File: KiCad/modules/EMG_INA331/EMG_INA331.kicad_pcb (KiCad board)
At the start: 4 copper layers, 15 x 11 mm, 47 parts, among them J1 Conn_01x01_Pin, J10 Conn_01x01_Pin, J2 Conn_01x01_Pin, J3 Conn_01x01_Pin, J4 Conn_01x01_Pin, J5 Conn_01x01_Pin, J6 Conn_01x01_Pin, J7 Conn_01x01_Pin, J8 Conn_01x01_Pin, J9 Conn_01x01_Pin, U1 INA350ABSIDSGR, U2 OPA333, U3 AP2112K-3.3TRG1, U4 OPA333, U5 CJ432, U6 LIS3DHTR

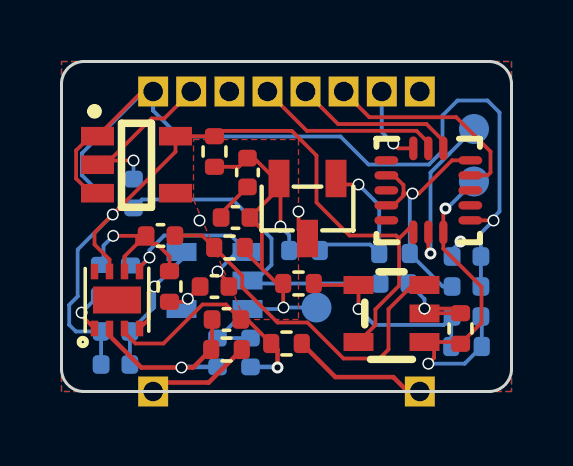
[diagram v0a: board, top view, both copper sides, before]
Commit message: cleaned all modules + production files
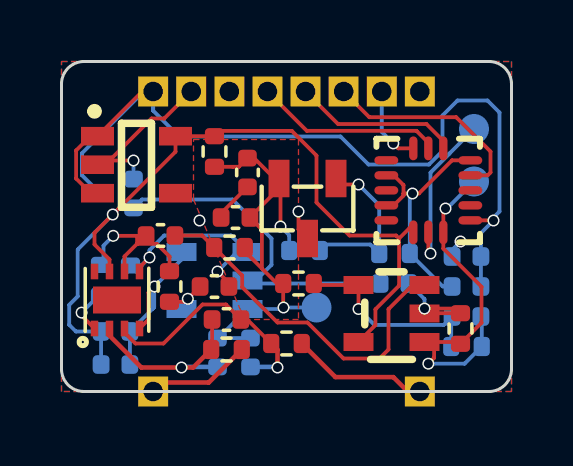
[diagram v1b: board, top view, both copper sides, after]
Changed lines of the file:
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@@
 		(sheetname "Root")
 		(sheetfile "EMG_INA331.kicad_sch")
-		(attr through_hole exclude_from_pos_files)
+		(attr through_hole exclude_from_pos_files exclude_from_bom dnp)
 		(fp_line
 			(start -1.05 -0.11)
@@
 			(size 1 1)
 			(drill 0.65)
+			(property pad_prop_castellated)
 			(layers "*.Cu" "*.Mask")
 			(remove_unused_layers no)
@@
 		(sheetname "Root")
 		(sheetfile "EMG_INA331.kicad_sch")
-		(attr through_hole exclude_from_pos_files)
+		(attr through_hole exclude_from_pos_files exclude_from_bom dnp)
 		(fp_line
 			(start -1.05 -0.11)
@@
 			(size 1 1)
 			(drill 0.65)
+			(property pad_prop_castellated)
 			(layers "*.Cu" "*.Mask")
 			(remove_unused_layers no)
@@
 		(at 35.8 32)
 		(size 0.4)
-		(drill 0.2)
+		(drill 0.3)
 		(layers "F.Cu" "B.Cu")
 		(net 1)
@@
 		(at 29.7 36.2)
 		(size 0.4)
-		(drill 0.2)
+		(drill 0.3)
 		(layers "F.Cu" "B.Cu")
 		(net 19)
@@
 		(at 35.3 30.9)
 		(size 0.4)
-		(drill 0.2)
+		(drill 0.3)
 		(layers "F.Cu" "B.Cu")
 		(net 22)
@@
 		(at 34.8 32.4)
 		(size 0.4)
-		(drill 0.2)
+		(drill 0.3)
 		(layers "F.Cu" "B.Cu")
 		(net 29)
